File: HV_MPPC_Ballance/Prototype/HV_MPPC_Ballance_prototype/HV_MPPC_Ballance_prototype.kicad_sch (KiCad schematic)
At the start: 9 parts, among them J1 HV_In, U9 ADP5600ACPZ-R7

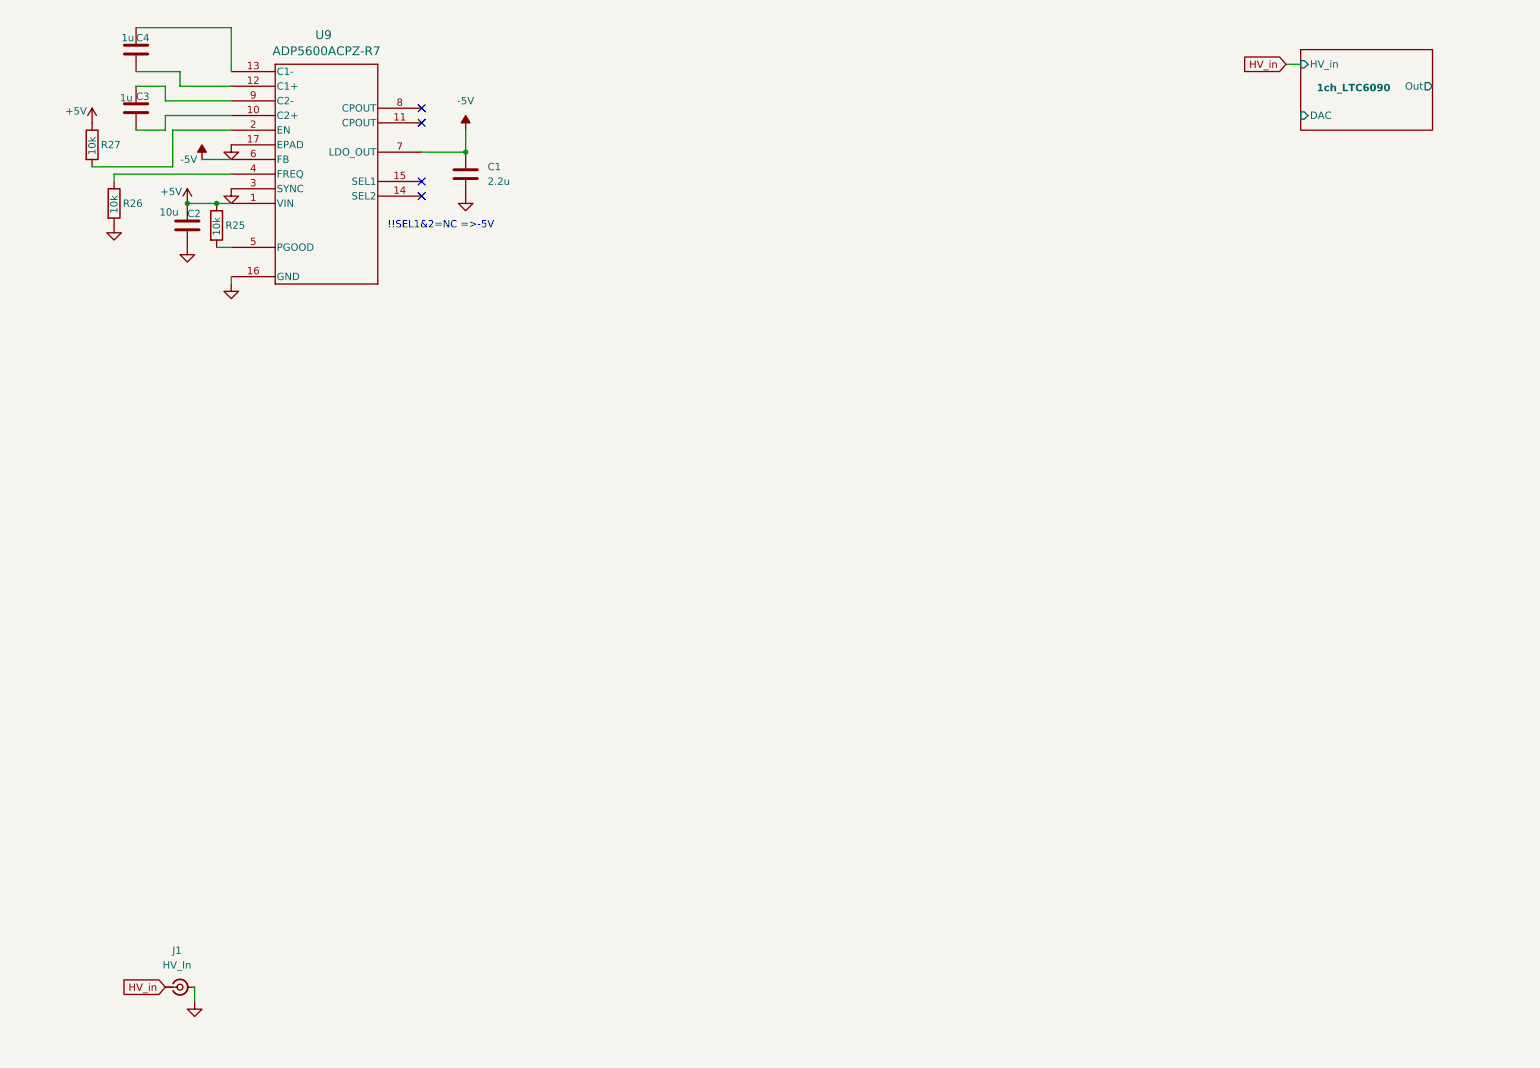
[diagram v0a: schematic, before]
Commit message: .
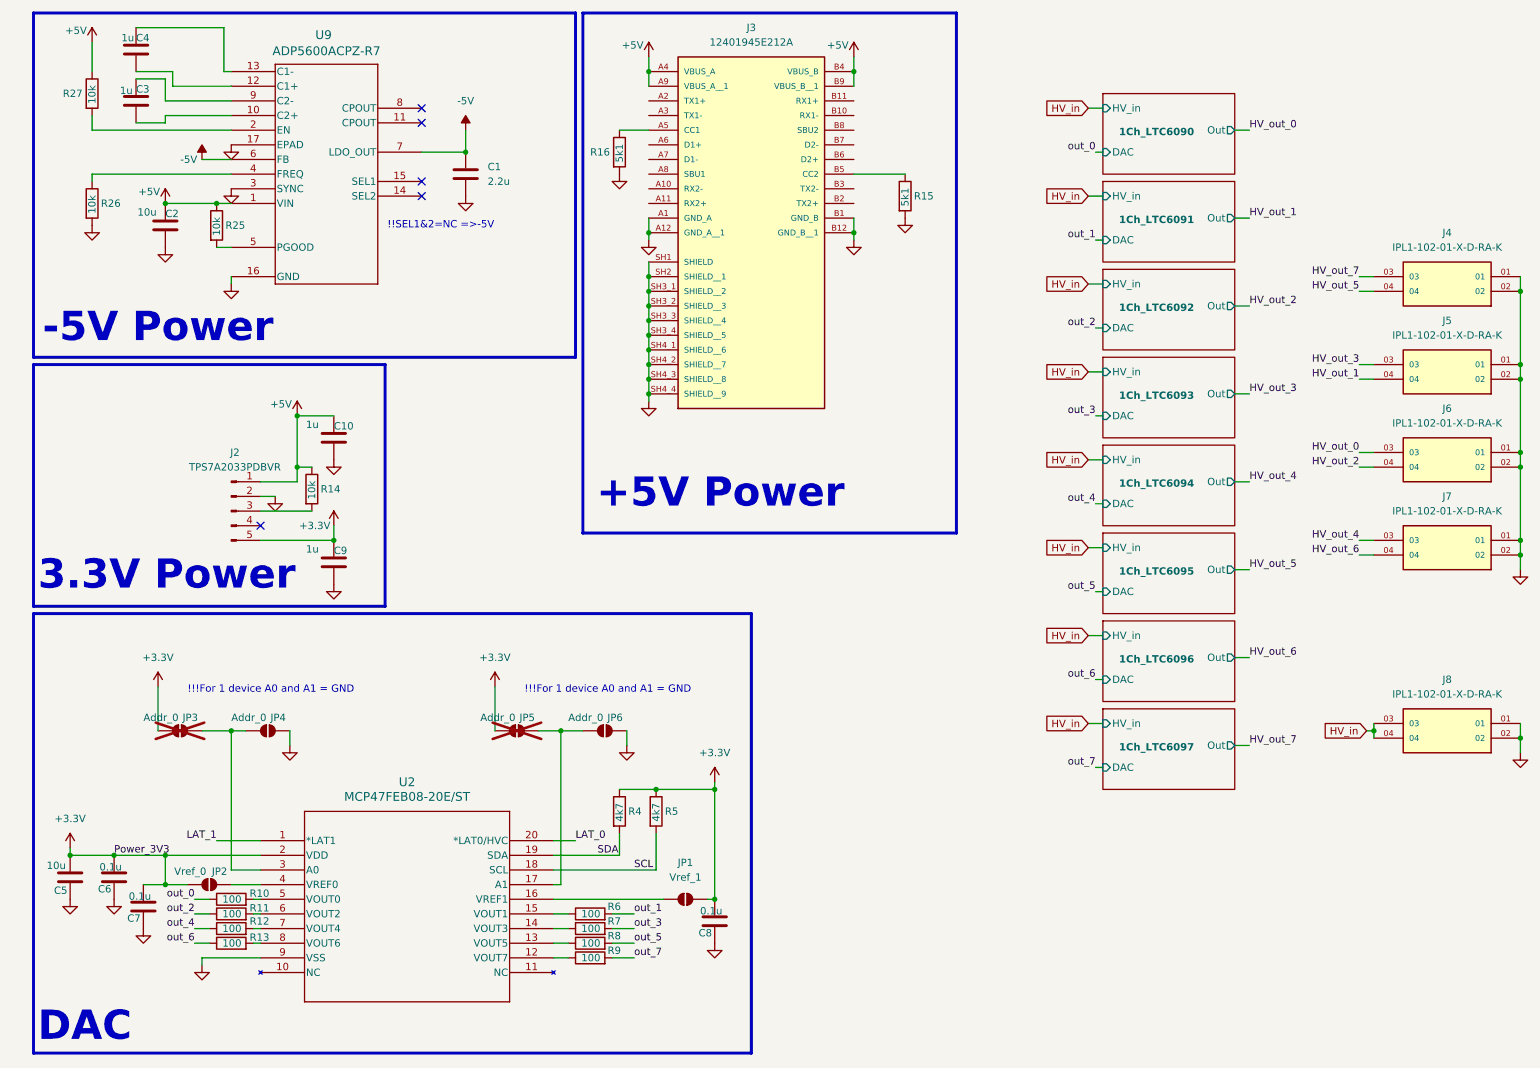
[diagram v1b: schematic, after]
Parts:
- removed J1: HV_In, symbol Connector:Conn_Coaxial_Small
- added C10, C9: 1u, Capacitor_SMD:C_0603_1608Metric, symbol Device:C
- added C5: 10u, Capacitor_SMD:C_0603_1608Metric, symbol Device:C
- added C6, C7, C8: 0.1u, Capacitor_SMD:C_0603_1608Metric, symbol Device:C
- added J2: TPS7A2033PDBVR, Package_TO_SOT_SMD:TSOT-23-5_HandSoldering, symbol Connector:Conn_01x05_Pin
- added J3: 12401945E212A, 0_lib:AMPHENOL_12401945E212A, symbol 0_lib:12401945E212A
- added J4, J5, J6, J7, J8: IPL1-102-01-X-D-RA-K, 0_lib:SAMTEC_IPL1-102-01-X-D-RA-K, symbol 0_lib:IPL1-102-01-X-D-RA-K
- added JP1: Vref_1, Jumper:SolderJumper-2_P1.3mm_Open_Pad1.0x1.5mm, symbol Jumper:SolderJumper_2_Open
- added JP2: Vref_0, Jumper:SolderJumper-2_P1.3mm_Open_Pad1.0x1.5mm, symbol Jumper:SolderJumper_2_Open
- added JP3, JP4, JP5, JP6: Addr_0, Jumper:SolderJumper-2_P1.3mm_Open_Pad1.0x1.5mm, symbol Jumper:SolderJumper_2_Open
- added R10, R11, R12, R13, R6, R7, R8, R9: 100, Resistor_SMD:R_0603_1608Metric, symbol Device:R
- added R14: 10k, Resistor_SMD:R_0603_1608Metric, symbol Device:R
- added R15, R16: 5k1, Resistor_SMD:R_0603_1608Metric, symbol Device:R
- added R4, R5: 4k7, Resistor_SMD:R_0603_1608Metric, symbol Device:R
- added U2: MCP47FEB08-20E/ST, 0_lib:TSSOP20_ST_MCH, symbol 0_lib:MCP47FVB28-20E_ST
- C1, C3, C4: footprint (none) -> Capacitor_SMD:C_0603_1608Metric
- C2: footprint (none) -> Capacitor_SMD:C_0805_2012Metric
- R25, R26, R27: footprint (none) -> Resistor_SMD:R_0603_1608Metric
- U9: footprint CP-16-17_ADI -> 0_lib:CP-16-17_ADI
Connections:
- net +5V: now also C10.1, J2.1 (Pin_1), J3.A4 (VBUS_A), J3.A9 (VBUS_A__1), J3.B4 (VBUS_B), J3.B9 (VBUS_B__1), R14.1
- net GND: now also C10.2, C5.2, C6.2, C7.2, C8.2, C9.2, J2.2 (Pin_2), J3.A1 (GND_A), J3.A12 (GND_A__1), J3.B1 (GND_B), J3.B12 (GND_B__1), J3.SH1 (SHIELD), J3.SH2 (SHIELD__1), J3.SH3_1 (SHIELD__2), J3.SH3_2 (SHIELD__3), J3.SH3_3 (SHIELD__4), J3.SH3_4 (SHIELD__5), J3.SH4_1 (SHIELD__6), J3.SH4_2 (SHIELD__7), J3.SH4_3 (SHIELD__8), J3.SH4_4 (SHIELD__9), J4.01, J4.02, J5.01, J5.02, J6.01, J6.02, J7.01, J7.02, J8.01, J8.02, JP4.2 (B), JP6.2 (B), R15.2, R16.2, U2.9 (VSS)
- net HV_in: now also J8.03, J8.04
- new net: JP3.2 (B), JP4.1 (A), U2.3 (A0)
- new net: R10.2, U2.5 (VOUT0)
- new net: J3.A5 (CC1), R16.1
- new net: R12.2, U2.7 (VOUT4)
- new net: J3.B5 (CC2), R15.1
- new net: JP1.1 (A), U2.16 (VREF1)
- new net: R13.2, U2.8 (VOUT6)
- new net: R11.2, U2.6 (VOUT2)
- new net: JP2.2 (B), U2.4 (VREF0)
- new net: R6.1, U2.15 (VOUT1)
- new net: R9.1, U2.12 (VOUT7)
- new net: R8.1, U2.13 (VOUT5)
- new net: R7.1, U2.14 (VOUT3)
- new net: JP5.2 (B), JP6.1 (A), U2.17 (A1)
- new net: J2.3 (Pin_3), R14.2
- new net +3.3V: C5.1, C6.1, C7.1, C8.1, C9.1, J2.5 (Pin_5), JP1.2 (B), JP2.1 (A), JP3.1 (A), JP5.1 (A), R4.1, R5.1, U2.2 (VDD)
- new net HV_out_0: J6.03
- new net HV_out_1: J5.04
- new net HV_out_2: J6.04
- new net HV_out_3: J5.03
- new net HV_out_4: J7.03
- new net HV_out_5: J4.04
- new net HV_out_6: J7.04
- new net HV_out_7: J4.03
- new net LAT_0: U2.20 (*LAT0/HVC)
- new net LAT_1: U2.1 (*LAT1)
- new net SCL: R5.2, U2.18 (SCL)
- new net SDA: R4.2, U2.19 (SDA)
- new net out_0: R10.1
- new net out_1: R6.2
- new net out_2: R11.1
- new net out_3: R7.2
- new net out_4: R12.1
- new net out_5: R8.2
- new net out_6: R13.1
- new net out_7: R9.2
- no-connect marks 4 -> 5
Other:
- sheet 1ch_LTC6090 renamed 1Ch_LTC6090
- added sheet 1Ch_LTC6091 (1_ch_ltc6090.kicad_sch)
- added sheet 1Ch_LTC6092 (1_ch_ltc6090.kicad_sch)
- added sheet 1Ch_LTC6093 (1_ch_ltc6090.kicad_sch)
- added sheet 1Ch_LTC6094 (1_ch_ltc6090.kicad_sch)
- added sheet 1Ch_LTC6095 (1_ch_ltc6090.kicad_sch)
- added sheet 1Ch_LTC6096 (1_ch_ltc6090.kicad_sch)
- added sheet 1Ch_LTC6097 (1_ch_ltc6090.kicad_sch)
- note added: "!!!For 1 device A0 and A1 = GND"
- note added: "+5V Power"
- note added: "-5V Power"
- note added: "3.3V Power"
- note added: "DAC"
- moved on the sheet: C2, C3, R26, R27
